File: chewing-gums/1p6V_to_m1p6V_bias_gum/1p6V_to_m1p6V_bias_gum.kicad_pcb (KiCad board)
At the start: 4 copper layers, 15.2 x 27.9 mm, 26 parts, among them J1 Conn_Coaxial, U1 LT1118, U2 TPS72301, U3 TLV75801PDBV, U4 MCP4726, U5 24AA02E-OT

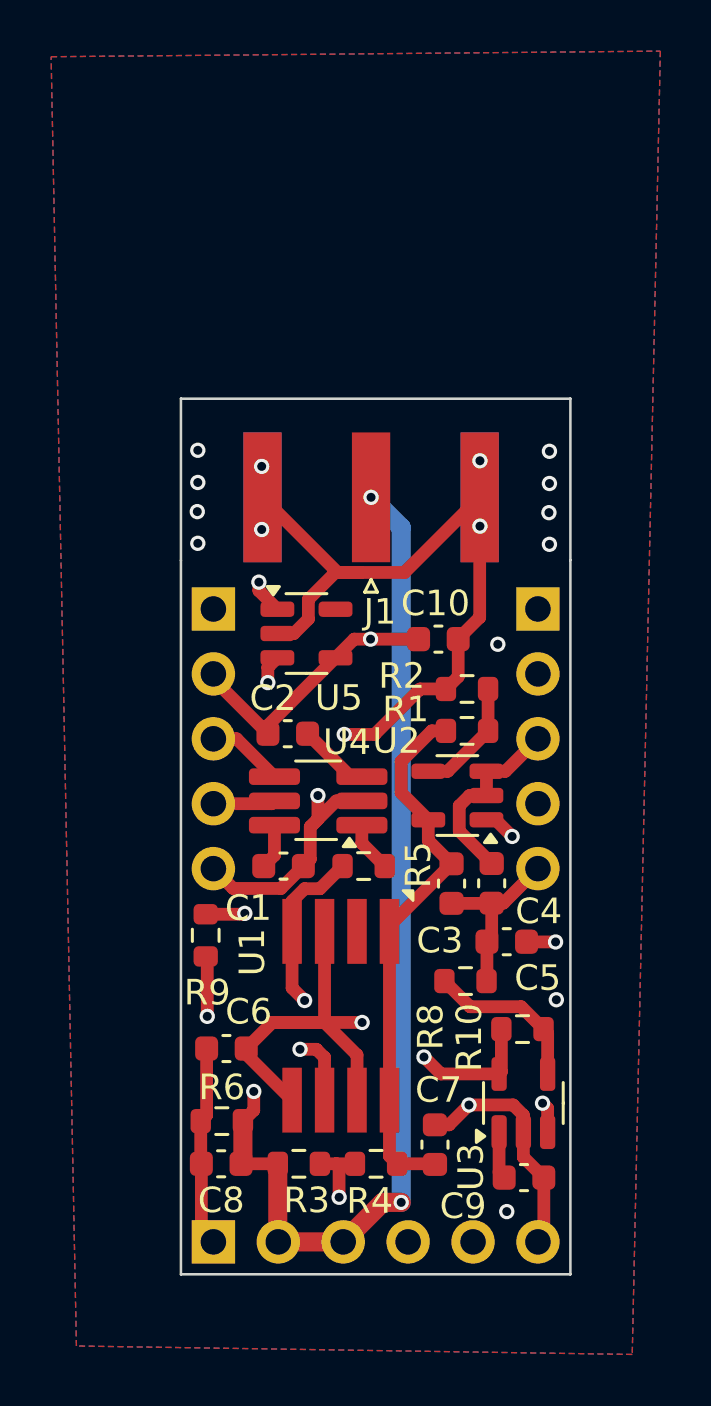
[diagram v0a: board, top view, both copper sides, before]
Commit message: production files
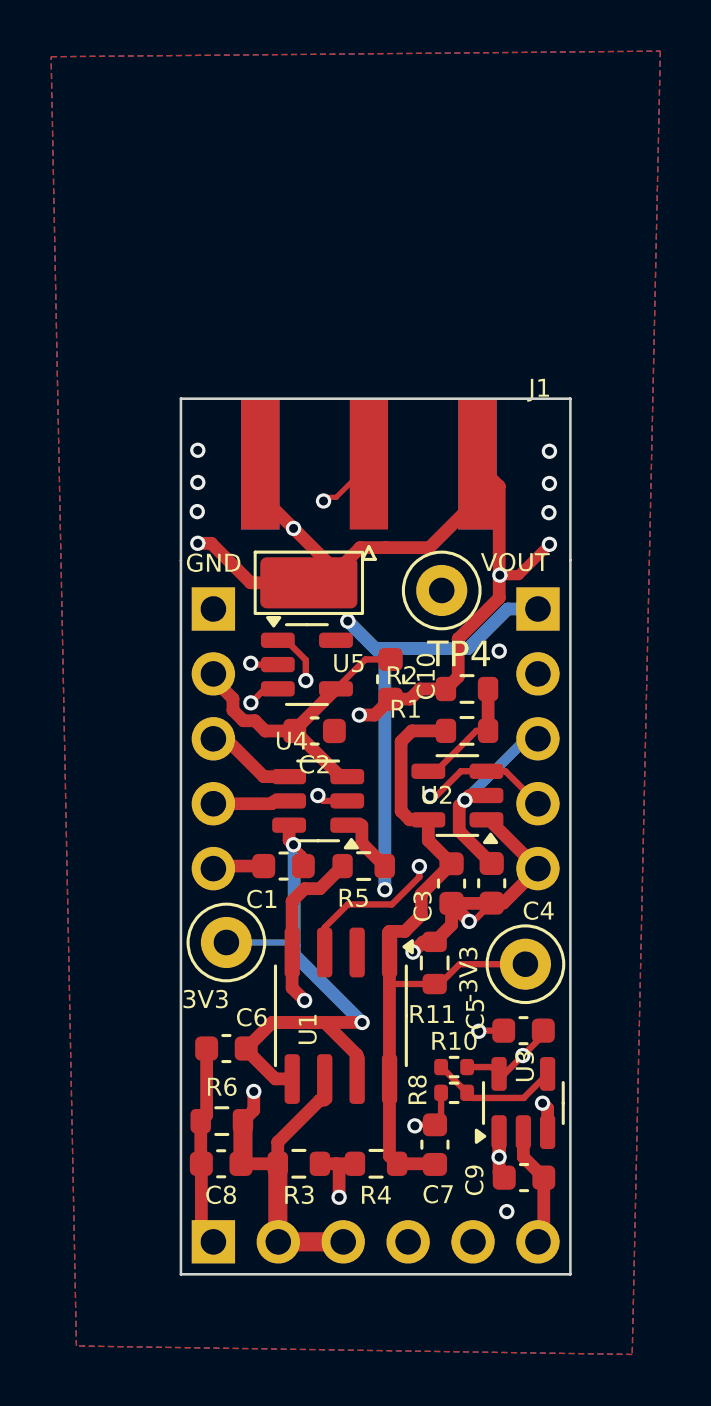
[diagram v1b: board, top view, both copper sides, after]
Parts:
- removed R9: 10k, Resistor_SMD:R_0603_1608Metric
- added G***: LOGO, heep-footprints:ESL_3x3, B.Cu at (84.2, 83.0)
- added G***: LOGO, heep-footprints:EPFL_3x1, B.Cu at (89.4, 76.8)
- added R11: 10k, Resistor_SMD:R_0603_1608Metric, F.Cu at (90.9, 76.0)
- added TP1: 5029, TestPoint:TestPoint_Loop_D1.80mm_Drill1.0mm_Beaded, F.Cu at (82.8, 75.2)
- added TP2: 5029, TestPoint:TestPoint_Loop_D1.80mm_Drill1.0mm_Beaded, F.Cu at (94.5, 76.0)
- added TP3: 5029, TestPoint:TestPoint_Keystone_5019_Miniature, F.Cu at (86.0, 61.1)
- added TP4: 5029, TestPoint:TestPoint_Loop_D1.80mm_Drill1.0mm_Beaded, F.Cu at (91.2, 61.4)
- C4, C6, C7, C9: value 1u -> 10u
- C5: value 1u -> 2.2u
- R10, R8: footprint Resistor_SMD:R_0603_1608Metric -> Resistor_SMD:R_0402_1005Metric
- R3, R5: value 33.2k -> 53.6k
- R4: value 7.03k -> 11.3k
- R6: value 1k -> 10k
- U1: footprint heep-footprints:S8-package -> Package_SO:SOIC-8_3.9x4.9mm_P1.27mm
- U4: footprint Package_TO_SOT_SMD:TSOT-23-6_HandSoldering -> Package_TO_SOT_SMD:TSOT-23-6
- moved R8 4.40 mm to (91.7, 81.1), turned to 180 degrees
- moved C5 3.54 mm to (94.4, 78.7)
- moved R10 3.06 mm to (91.7, 80.1), turned to 180 degrees
- moved C10 2.44 mm to (89.2, 64.9), turned to -90 degrees
- moved J1 1.28 mm to (88.3, 56.5)
- moved U5 1.22 mm to (85.9, 64.3)
- moved C2 1.06 mm to (86.2, 66.9), turned to 0 degrees
- moved U1 0.07 mm to (87.2, 78.1)
- turned C1 to 180 degrees
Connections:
- C1 pad 1: Net-(U4-Vref) -> /3.3VA
- C10 pad 1: 3.3V -> /3.3V
- C2 pad 1: Net-(U4-VDD) -> /3.3V
- C2 pad 2: 3.3V -> GND
- C5 pad 1: Net-(U2-GND) -> /3.3VA
- C9 pad 1: Net-(U3-IN) -> /5V
- CG1 pad A1: unconnected-(CG1-5V-PadA1) -> /5V
- CG1 pad A2: 3.3V -> /3.3V
- CG1 pad B1: unconnected-(CG1-5V-PadB1) -> /5V
- CG1 pad B4: unconnected-(CG1-ENABLE-PadB4) -> /enable
- U1 pad 3: /3.3VA -> /enable
- U2 pad 1: Net-(U2-GND) -> GND
- U2 pad 3: /-5V -> /enable
- U3 pad 1: Net-(U3-IN) -> /5V
- U3 pad 3: Net-(U3-EN) -> /enable
- U4 pad 3: Net-(U4-VDD) -> /3.3V
- U4 pad 6: Net-(U4-Vref) -> /3.3VA
- U5 pad 4: 3.3V -> /3.3V
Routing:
- net /5V: track 0.00 -> 40.6 mm, vias 0 -> 3
- net /enable: track 0.00 -> 27.8 mm, vias 0 -> 3
- net 3.3V: track 25.2 -> 0.00 mm, vias 2 -> 0
- net Net-(U3-EN): track 19.2 -> 0.00 mm, vias 2 -> 0
- net /3.3V: track 0.00 -> 12.2 mm
- net /3.3VA: track 24.9 -> 35.6 mm, vias 2 -> 3
- net Net-(U2-GND): track 7.45 -> 0.00 mm, vias 2 -> 0
- net GND: track 65.1 -> 72.5 mm, vias 18 -> 19
- net /-3.3VA: track 21.4 -> 28.3 mm
- net /SCL: track 14.7 -> 11.0 mm
- net /V_bias: track 46.3 -> 49.9 mm, vias 4 -> 2
- net Net-(U4-VDD): track 2.82 -> 0.00 mm
- net Net-(U4-Vref): track 1.92 -> 0.00 mm
- net Net-(U3-IN): track 1.86 -> 0.00 mm
- net Net-(U3-FB): track 6.48 -> 5.06 mm
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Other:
- board text added: "+/-1.5V programmable Supply ESL 2025"
- board text added: "-3V3"
- board text added: "3V3"
- board text added: "GND"
- board text added: "VOUT"
